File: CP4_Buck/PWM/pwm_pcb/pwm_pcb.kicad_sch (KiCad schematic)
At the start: 11 parts, among them J1 in, J2 ref, J3 out, U2 LM324, U3 LTC6702CDC_PBF

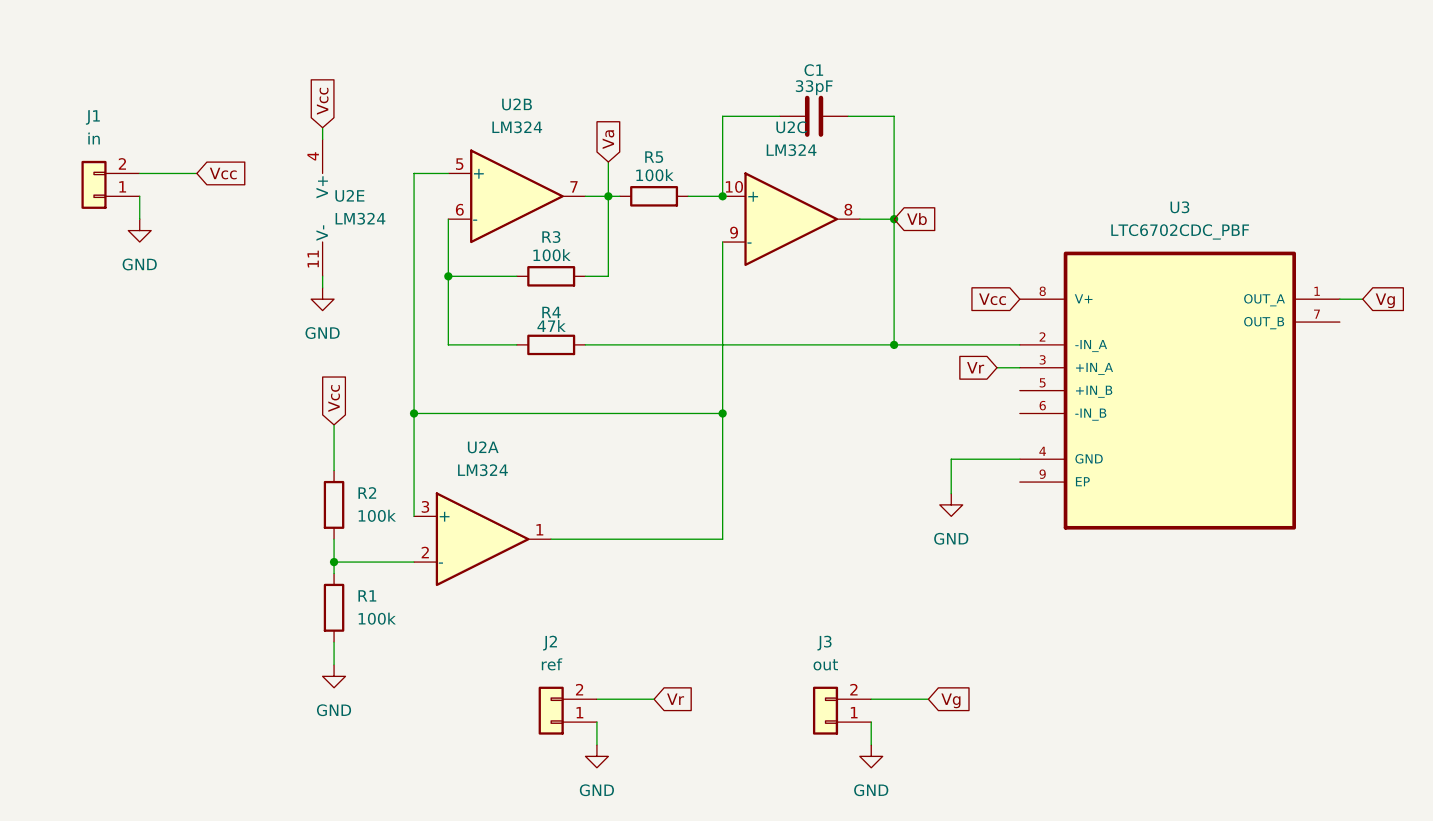
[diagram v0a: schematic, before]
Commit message: Add files via upload
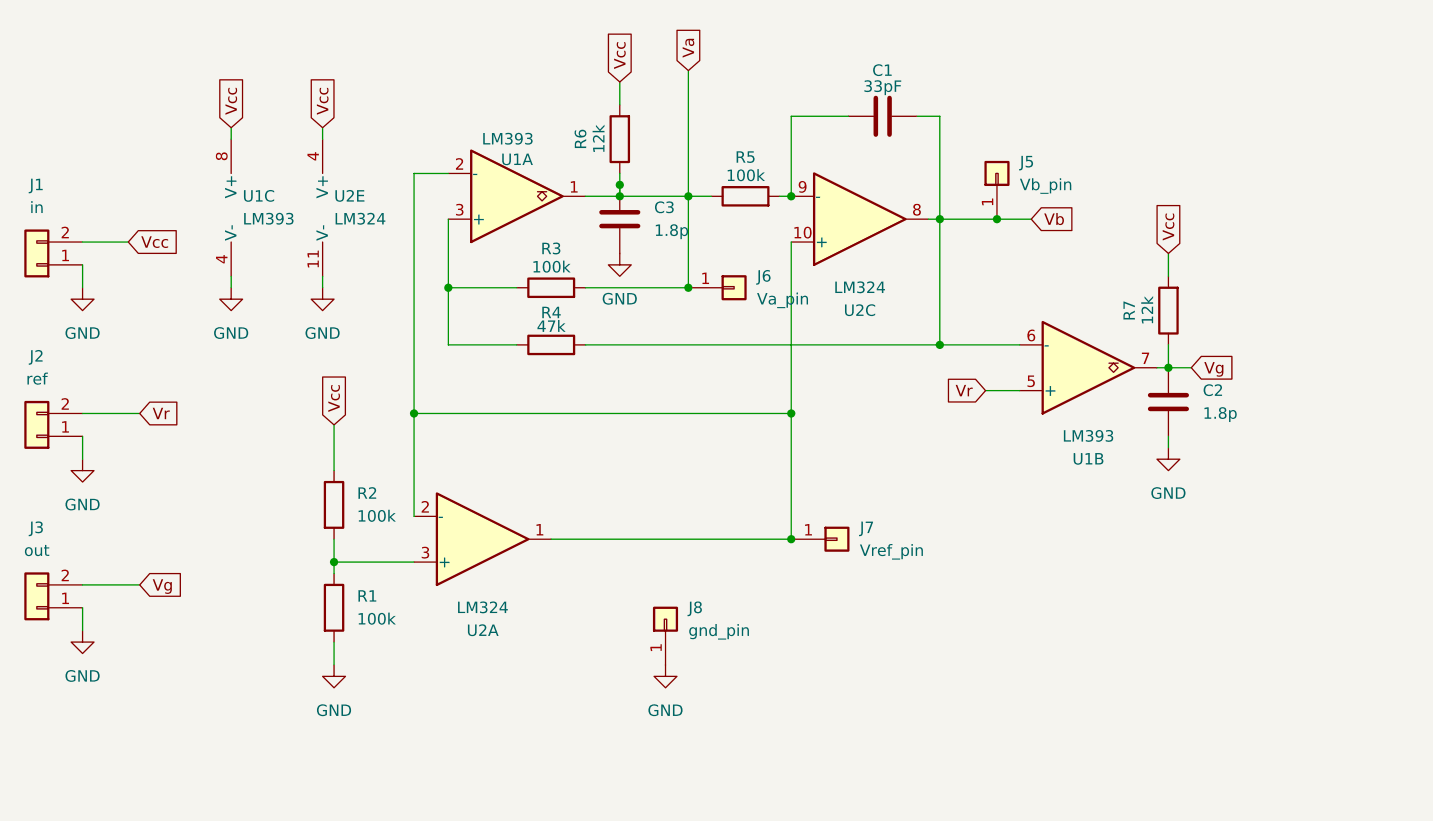
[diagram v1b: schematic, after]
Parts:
- removed unit 2 of U2
- removed U3: LTC6702CDC_PBF, LTC6702CTS8_TRMPBF:SOT65P280X100-8N, symbol LTC6702CDC_PBF:LTC6702CDC_PBF
- added C2, C3: 1.8p, Capacitor_THT:C_Disc_D3.0mm_W1.6mm_P2.50mm, symbol Device:C
- added J5: Vb_pin, Connector_PinHeader_2.54mm:PinHeader_1x01_P2.54mm_Vertical, symbol Connector_Generic:Conn_01x01
- added J6: Va_pin, Connector_PinHeader_2.54mm:PinHeader_1x01_P2.54mm_Vertical, symbol Connector_Generic:Conn_01x01
- added J7: Vref_pin, Connector_PinHeader_2.54mm:PinHeader_1x01_P2.54mm_Vertical, symbol Connector_Generic:Conn_01x01
- added J8: gnd_pin, Connector_PinHeader_2.54mm:PinHeader_1x01_P2.54mm_Vertical, symbol Connector_Generic:Conn_01x01
- added R6, R7: 12k, Resistor_THT:R_Axial_DIN0204_L3.6mm_D1.6mm_P5.08mm_Horizontal, symbol Device:R
- added U1: LM393, Package_DIP:DIP-8_W7.62mm, symbol Comparator:LM393
- R4: footprint Potentiometer_THT:Potentiometer_Bourns_3296W_Vertical -> Resistor_THT:R_Axial_DIN0204_L3.6mm_D1.6mm_P5.08mm_Horizontal
- R5: footprint Resistor_THT:R_Axial_DIN0204_L3.6mm_D1.6mm_P5.08mm_Horizontal -> Potentiometer_THT:Potentiometer_Bourns_3296W_Vertical
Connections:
- net GND: now also C2.2, C3.2, J8.1 (Pin_1), U1.4 (V-)
- net Va: now also C3.1, J6.1 (Pin_1), R6.1, U1.1
- net Vb: now also J5.1 (Pin_1), U1.6 (-)
- net Vcc: now also R6.2, R7.2, U1.8 (V+)
- net Vg: now also C2.1, R7.1, U1.7
- net Vr: now also U1.5 (+)
- net at R1.1, R2.2: now also U2.3 (+); no longer U2.2 (-)
- net at R3.1, R4.1: now also U1.3 (+)
- net at C1.1, R5.2: now also U2.9 (-); no longer U2.10 (+)
- new net: J7.1 (Pin_1), U1.2 (-), U2.1, U2.10 (+), U2.2 (-)
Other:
- moved on the sheet: C1, J1, J2, J3, R3, R5, U2C
